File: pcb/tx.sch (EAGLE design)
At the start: 51 parts, among them U3 MCP73831T-2ACI/OT, Y1 CRYSTAL-26MHZSMD-3.2X2.5

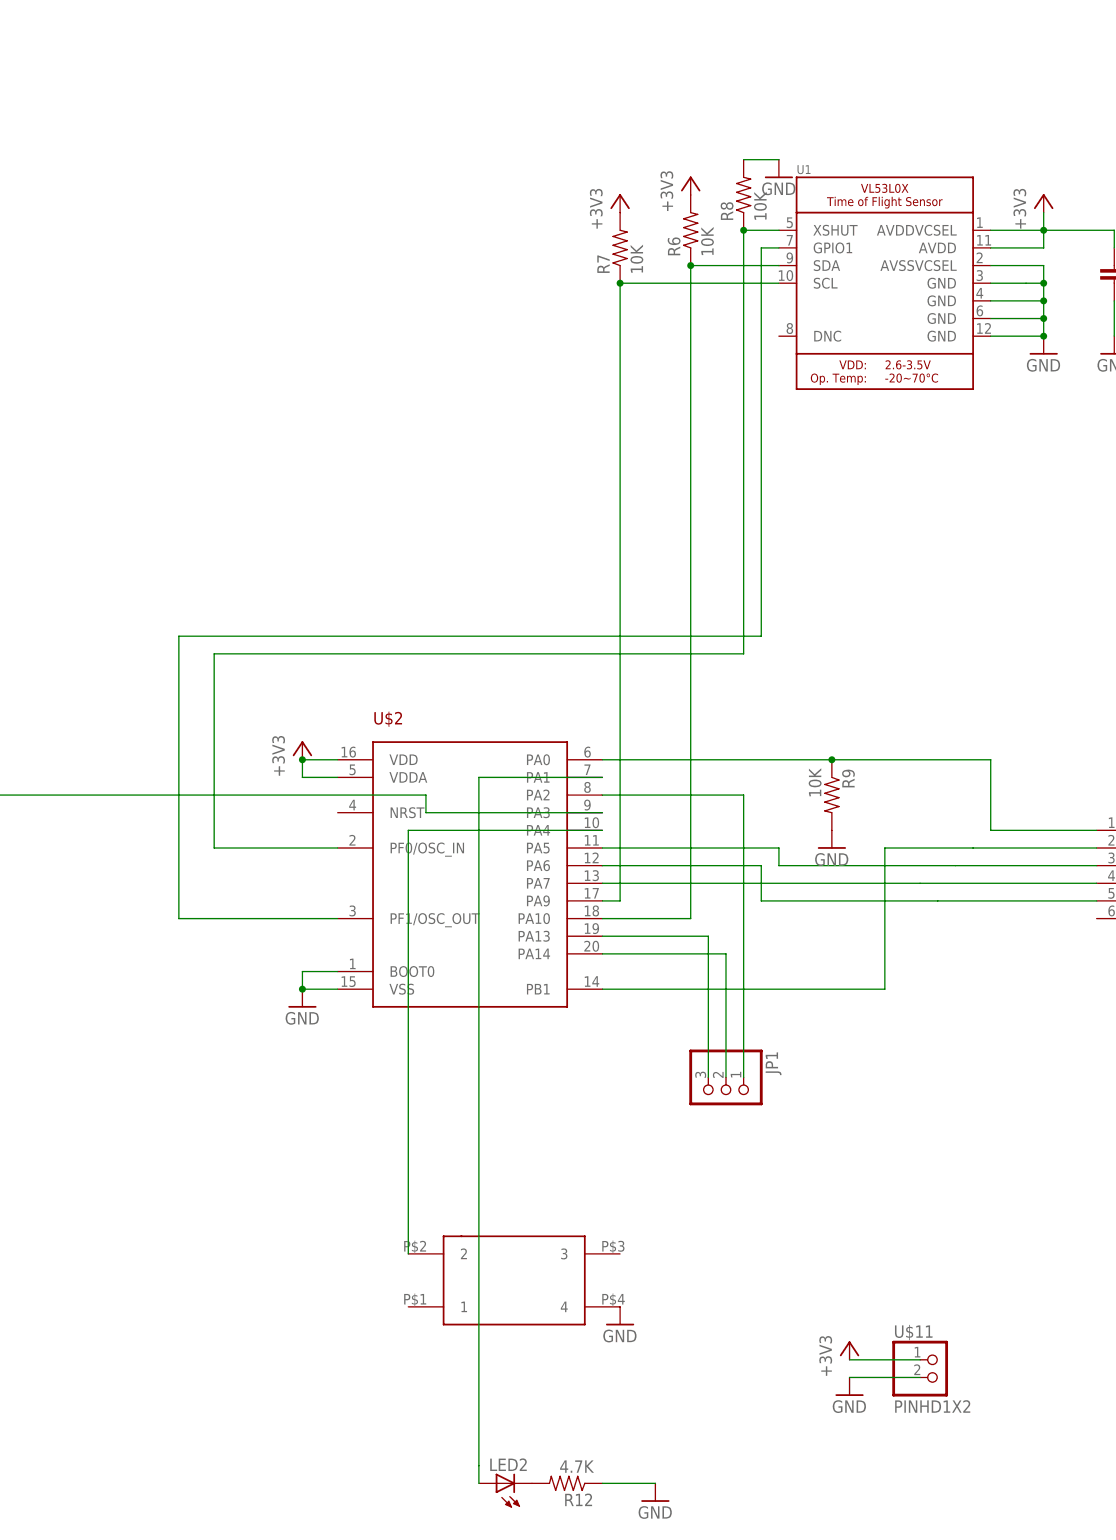
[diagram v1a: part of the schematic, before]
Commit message: further cleanup
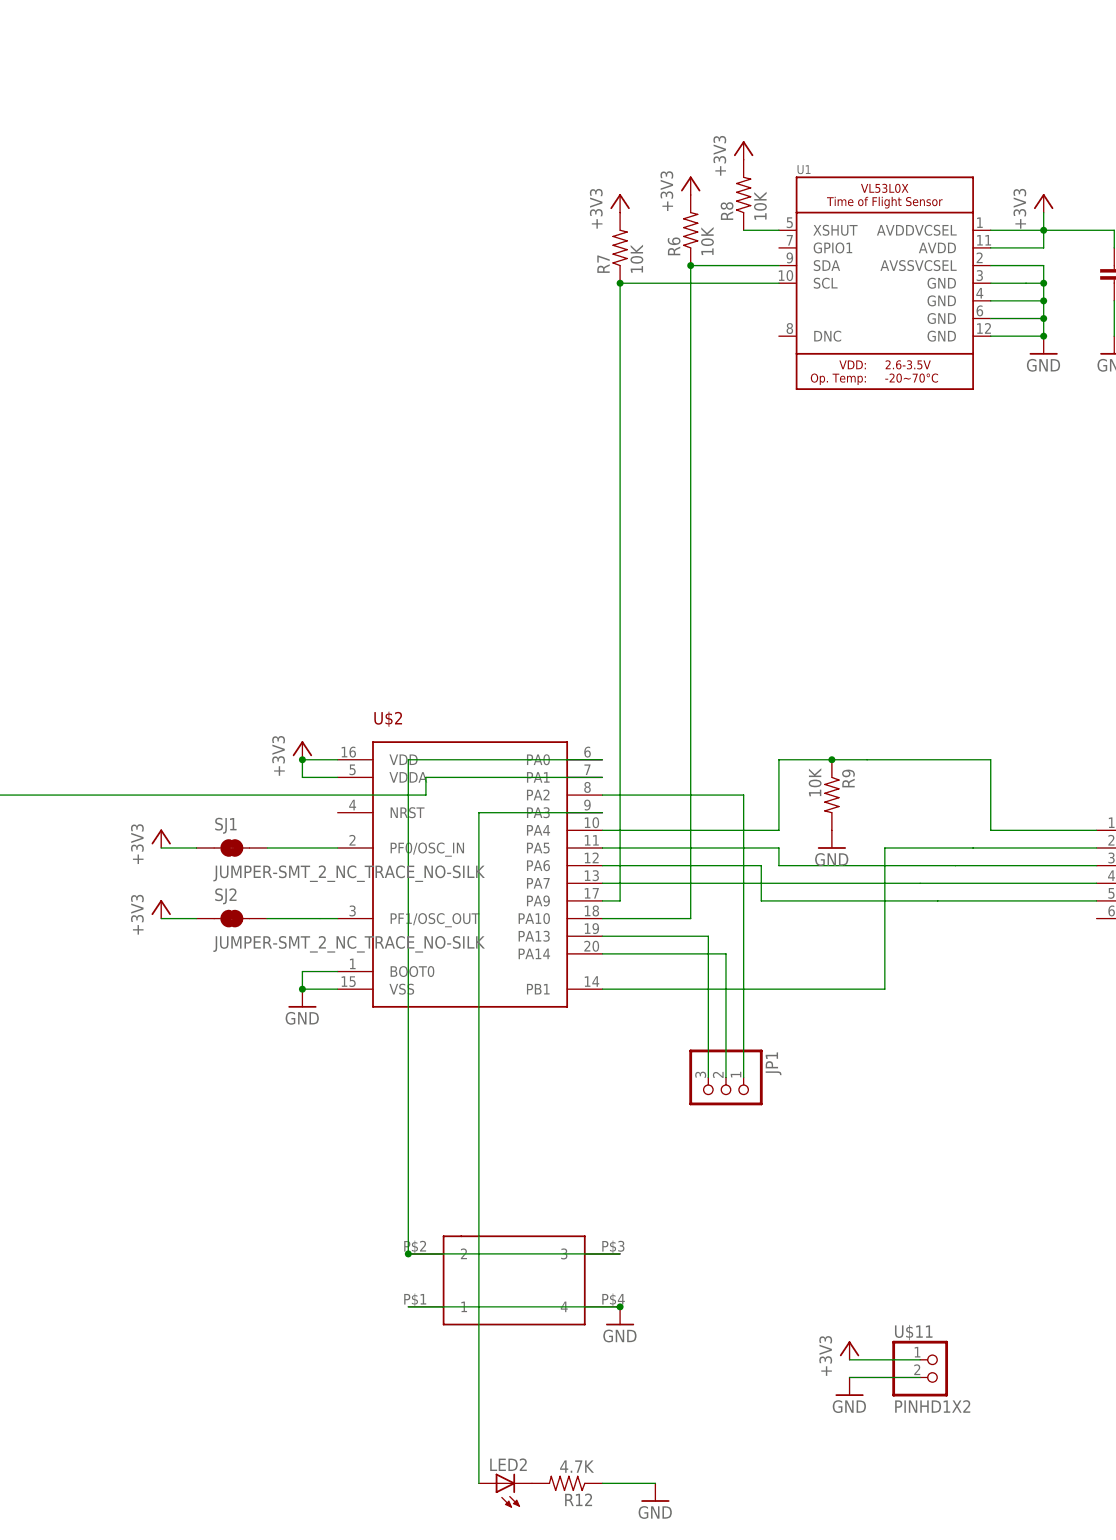
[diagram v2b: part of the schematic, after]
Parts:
- added SJ1, SJ2: JUMPER-SMT_2_NC_TRACE_NO-SILK, SparkFun-Jumpers:JUMPER-SMT_2_NC_TRACE_NO-SILK
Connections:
- new net N$34: SJ2.2, U$2.PF1/OSC_OUT
- net +3V3: now also R8.2, SJ1.1, SJ2.1
- net GND: now also U$10.1; no longer R8.2
- net N$21: now also U$2.PA4; no longer U$2.PA0
- net N$23: now also SJ1.2; no longer R8.1, U1.XSHUT
- net N$24: now also R8.1, U1.XSHUT; no longer U$2.PF1/OSC_OUT, U1.GPIO1
- net N$29: now also U$2.PA3; no longer U$2.PA1
- net N$30: now also U$10.3, U$2.PA0; no longer U$2.PA4
- net N$35: now also U$2.PA1; no longer U$2.PA3
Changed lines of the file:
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@@
 <part name="R9" library="joyAnalog" deviceset="RESISTOR" device="0805-RES" value="10K"/>
 <part name="GND25" library="supply1" library_urn="urn:adsk.eagle:library:371" deviceset="GND" device=""/>
-<part name="GND26" library="clock" deviceset="GND" device=""/>
 <part name="LED2" library="joyAnalog" deviceset="LED" device="CHIP-LED0805"/>
 <part name="R12" library="joyAnalog" deviceset="RESISTOR" device="0805-RES" value="4.7K"/>
@@
 <part name="GND30" library="supply1" library_urn="urn:adsk.eagle:library:371" deviceset="GND" device=""/>
 <part name="JP1" library="adafruit_changed" deviceset="PINHD-1X3" device="CB"/>
+<part name="+3V8" library="supply1" library_urn="urn:adsk.eagle:library:371" deviceset="+3V3" device=""/>
+<part name="SJ1" library="SparkFun-Jumpers" deviceset="JUMPER-SMT_2_NC_TRACE" device="_NO-SILK"/>
+<part name="SJ2" library="SparkFun-Jumpers" deviceset="JUMPER-SMT_2_NC_TRACE" device="_NO-SILK"/>
+<part name="+3V9" library="supply1" library_urn="urn:adsk.eagle:library:371" deviceset="+3V3" device=""/>
+<part name="+3V10" library="supply1" library_urn="urn:adsk.eagle:library:371" deviceset="+3V3" device=""/>
 </parts>
 <sheets>
@@
 <instance part="R9" gate="G$1" x="38.1" y="-48.26" rot="R270"/>
 <instance part="GND25" gate="1" x="38.1" y="-55.88"/>
-<instance part="GND26" gate="1" x="30.48" y="40.64"/>
 <instance part="LED2" gate="G$1" x="-10.16" y="-147.32" rot="R90"/>
 <instance part="R12" gate="G$1" x="0" y="-147.32" rot="R180"/>
@@
 <instance part="GND30" gate="1" x="-162.56" y="-71.12"/>
 <instance part="JP1" gate="A" x="22.86" y="-91.44" rot="R270"/>
+<instance part="+3V8" gate="G$1" x="25.4" y="45.72"/>
+<instance part="SJ1" gate="G$1" x="-48.26" y="-55.88"/>
+<instance part="SJ2" gate="G$1" x="-48.26" y="-66.04"/>
+<instance part="+3V9" gate="G$1" x="-58.42" y="-53.34"/>
+<instance part="+3V10" gate="G$1" x="-58.42" y="-63.5"/>
 </instances>
 <busses>
@@
 </segment>
 <segment>
-<pinref part="GND26" gate="1" pin="GND"/>
-<pinref part="R8" gate="G$1" pin="2"/>
-<wire x1="30.48" y1="43.18" x2="25.4" y2="43.18" width="0.1524" layer="91"/>
-</segment>
-<segment>
 <pinref part="U$10" gate="G$1" pin="4"/>
 <pinref part="GND27" gate="1" pin="GND"/>
+<pinref part="U$10" gate="G$1" pin="1"/>
+<wire x1="7.62" y1="-121.92" x2="-22.86" y2="-121.92" width="0.1524" layer="91"/>
+<junction x="7.62" y="-121.92"/>
 </segment>
 <segment>
@@
 <wire x1="40.64" y1="-129.54" x2="50.8" y2="-129.54" width="0.1524" layer="91"/>
 </segment>
+<segment>
+<pinref part="R8" gate="G$1" pin="2"/>
+<pinref part="+3V8" gate="G$1" pin="+3V3"/>
+</segment>
+<segment>
+<pinref part="+3V9" gate="G$1" pin="+3V3"/>
+<pinref part="SJ1" gate="G$1" pin="1"/>
+<wire x1="-58.42" y1="-55.88" x2="-53.34" y2="-55.88" width="0.1524" layer="91"/>
+</segment>
+<segment>
+<pinref part="+3V10" gate="G$1" pin="+3V3"/>
+<pinref part="SJ2" gate="G$1" pin="1"/>
+<wire x1="-58.42" y1="-66.04" x2="-53.34" y2="-66.04" width="0.1524" layer="91"/>
+</segment>
 </net>
 <net name="N$1" class="0">
@@
 <pinref part="U$3" gate="G$1" pin="CE"/>
 <wire x1="76.2" y1="-53.34" x2="60.96" y2="-53.34" width="0.1524" layer="91"/>
-<pinref part="U$2" gate="G$1" pin="PA0"/>
 <wire x1="60.96" y1="-53.34" x2="60.96" y2="-43.18" width="0.1524" layer="91"/>
-<wire x1="60.96" y1="-43.18" x2="38.1" y2="-43.18" width="0.1524" layer="91"/>
+<wire x1="60.96" y1="-43.18" x2="43.18" y2="-43.18" width="0.1524" layer="91"/>
 <pinref part="R9" gate="G$1" pin="1"/>
-<wire x1="38.1" y1="-43.18" x2="5.08" y2="-43.18" width="0.1524" layer="91"/>
+<wire x1="43.18" y1="-43.18" x2="38.1" y2="-43.18" width="0.1524" layer="91"/>
+<pinref part="U$2" gate="G$1" pin="PA4"/>
+<wire x1="5.08" y1="-53.34" x2="30.48" y2="-53.34" width="0.1524" layer="91"/>
+<wire x1="30.48" y1="-53.34" x2="30.48" y2="-43.18" width="0.1524" layer="91"/>
+<wire x1="30.48" y1="-43.18" x2="38.1" y2="-43.18" width="0.1524" layer="91"/>
 <junction x="38.1" y="-43.18"/>
 </segment>
@@
 </segment>
 </net>
-<net name="N$23" class="0">
-<segment>
-<pinref part="U1" gate="G$1" pin="XSHUT"/>
-<pinref part="R8" gate="G$1" pin="1"/>
-<wire x1="30.48" y1="33.02" x2="25.4" y2="33.02" width="0.1524" layer="91"/>
-<wire x1="25.4" y1="33.02" x2="25.4" y2="-27.94" width="0.1524" layer="91"/>
-<wire x1="25.4" y1="-27.94" x2="-50.8" y2="-27.94" width="0.1524" layer="91"/>
-<junction x="25.4" y="33.02"/>
-<pinref part="U$2" gate="G$1" pin="PF0/OSC_IN"/>
-<wire x1="-50.8" y1="-27.94" x2="-50.8" y2="-55.88" width="0.1524" layer="91"/>
-<wire x1="-50.8" y1="-55.88" x2="-33.02" y2="-55.88" width="0.1524" layer="91"/>
-</segment>
-</net>
-<net name="N$24" class="0">
-<segment>
-<pinref part="U1" gate="G$1" pin="GPIO1"/>
-<wire x1="30.48" y1="30.48" x2="27.94" y2="30.48" width="0.1524" layer="91"/>
-<wire x1="27.94" y1="30.48" x2="27.94" y2="-25.4" width="0.1524" layer="91"/>
-<wire x1="27.94" y1="-25.4" x2="-55.88" y2="-25.4" width="0.1524" layer="91"/>
-<pinref part="U$2" gate="G$1" pin="PF1/OSC_OUT"/>
-<wire x1="-55.88" y1="-25.4" x2="-55.88" y2="-66.04" width="0.1524" layer="91"/>
-<wire x1="-55.88" y1="-66.04" x2="-33.02" y2="-66.04" width="0.1524" layer="91"/>
-</segment>
-</net>
 <net name="N$28" class="0">
 <segment>
 <pinref part="LED2" gate="G$1" pin="C"/>
 <pinref part="R12" gate="G$1" pin="2"/>
-</segment>
-</net>
-<net name="N$29" class="0">
-<segment>
-<pinref part="U$2" gate="G$1" pin="PA1"/>
-<wire x1="5.08" y1="-45.72" x2="-12.7" y2="-45.72" width="0.1524" layer="91"/>
-<wire x1="-12.7" y1="-45.72" x2="-12.7" y2="-144.78" width="0.1524" layer="91"/>
-<pinref part="LED2" gate="G$1" pin="A"/>
-<wire x1="-12.7" y1="-144.78" x2="-12.7" y2="-147.32" width="0.1524" layer="91"/>
-</segment>
-</net>
-<net name="N$30" class="0">
-<segment>
-<pinref part="U$2" gate="G$1" pin="PA4"/>
-<wire x1="5.08" y1="-53.34" x2="-12.7" y2="-53.34" width="0.1524" layer="91"/>
-<pinref part="U$10" gate="G$1" pin="2"/>
-<wire x1="-12.7" y1="-53.34" x2="-22.86" y2="-53.34" width="0.1524" layer="91"/>
-<wire x1="-22.86" y1="-53.34" x2="-22.86" y2="-114.3" width="0.1524" layer="91"/>
 </segment>
 </net>
@@
 <pinref part="R11" gate="G$1" pin="2"/>
 <wire x1="-162.56" y1="-55.88" x2="-162.56" y2="-53.34" width="0.1524" layer="91"/>
-<pinref part="U$2" gate="G$1" pin="PA3"/>
 <wire x1="-162.56" y1="-53.34" x2="-162.56" y2="-48.26" width="0.1524" layer="91"/>
-<wire x1="5.08" y1="-50.8" x2="-20.32" y2="-50.8" width="0.1524" layer="91"/>
-<wire x1="-20.32" y1="-50.8" x2="-20.32" y2="-48.26" width="0.1524" layer="91"/>
+<wire x1="-152.4" y1="-53.34" x2="-162.56" y2="-53.34" width="0.1524" layer="91"/>
+<junction x="-162.56" y="-53.34"/>
+<pinref part="U$2" gate="G$1" pin="PA1"/>
+<wire x1="5.08" y1="-45.72" x2="-20.32" y2="-45.72" width="0.1524" layer="91"/>
+<wire x1="-20.32" y1="-45.72" x2="-20.32" y2="-48.26" width="0.1524" layer="91"/>
 <wire x1="-20.32" y1="-48.26" x2="-152.4" y2="-48.26" width="0.1524" layer="91"/>
 <wire x1="-152.4" y1="-48.26" x2="-152.4" y2="-53.34" width="0.1524" layer="91"/>
-<wire x1="-152.4" y1="-53.34" x2="-162.56" y2="-53.34" width="0.1524" layer="91"/>
-<junction x="-162.56" y="-53.34"/>
 </segment>
 </net>
@@
 </segment>
 </net>
+<net name="N$24" class="0">
+<segment>
+<pinref part="R8" gate="G$1" pin="1"/>
+<pinref part="U1" gate="G$1" pin="XSHUT"/>
+<wire x1="30.48" y1="33.02" x2="25.4" y2="33.02" width="0.1524" layer="91"/>
+</segment>
+</net>
+<net name="N$23" class="0">
+<segment>
+<pinref part="U$2" gate="G$1" pin="PF0/OSC_IN"/>
+<pinref part="SJ1" gate="G$1" pin="2"/>
+<wire x1="-33.02" y1="-55.88" x2="-43.18" y2="-55.88" width="0.1524" layer="91"/>
+</segment>
+</net>
+<net name="N$34" class="0">
+<segment>
+<pinref part="SJ2" gate="G$1" pin="2"/>
+<wire x1="-43.18" y1="-66.04" x2="-35.56" y2="-66.04" width="0.1524" layer="91"/>
+<pinref part="U$2" gate="G$1" pin="PF1/OSC_OUT"/>
+<wire x1="-35.56" y1="-66.04" x2="-33.02" y2="-66.04" width="0.1524" layer="91"/>
+</segment>
+</net>
+<net name="N$29" class="0">
+<segment>
+<pinref part="U$2" gate="G$1" pin="PA3"/>
+<pinref part="LED2" gate="G$1" pin="A"/>
+<wire x1="5.08" y1="-50.8" x2="-12.7" y2="-50.8" width="0.1524" layer="91"/>
+<wire x1="-12.7" y1="-50.8" x2="-12.7" y2="-147.32" width="0.1524" layer="91"/>
+</segment>
+</net>
+<net name="N$30" class="0">
+<segment>
+<pinref part="U$2" gate="G$1" pin="PA0"/>
+<pinref part="U$10" gate="G$1" pin="2"/>
+<wire x1="5.08" y1="-43.18" x2="-22.86" y2="-43.18" width="0.1524" layer="91"/>
+<wire x1="-22.86" y1="-43.18" x2="-22.86" y2="-114.3" width="0.1524" layer="91"/>
+<pinref part="U$10" gate="G$1" pin="3"/>
+<wire x1="-22.86" y1="-114.3" x2="7.62" y2="-114.3" width="0.1524" layer="91"/>
+<junction x="-22.86" y="-114.3"/>
+</segment>
+</net>
